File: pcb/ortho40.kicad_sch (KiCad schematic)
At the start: 128 parts, among them J1 SWD, J2 USB_C_Receptacle_USB2.0, SW1 SW_Push, U1 RP2040, U2 W25Q128JVS, U3 XC6206PxxxMR, U4 USBLC6-2SC6, Y1 12MHz

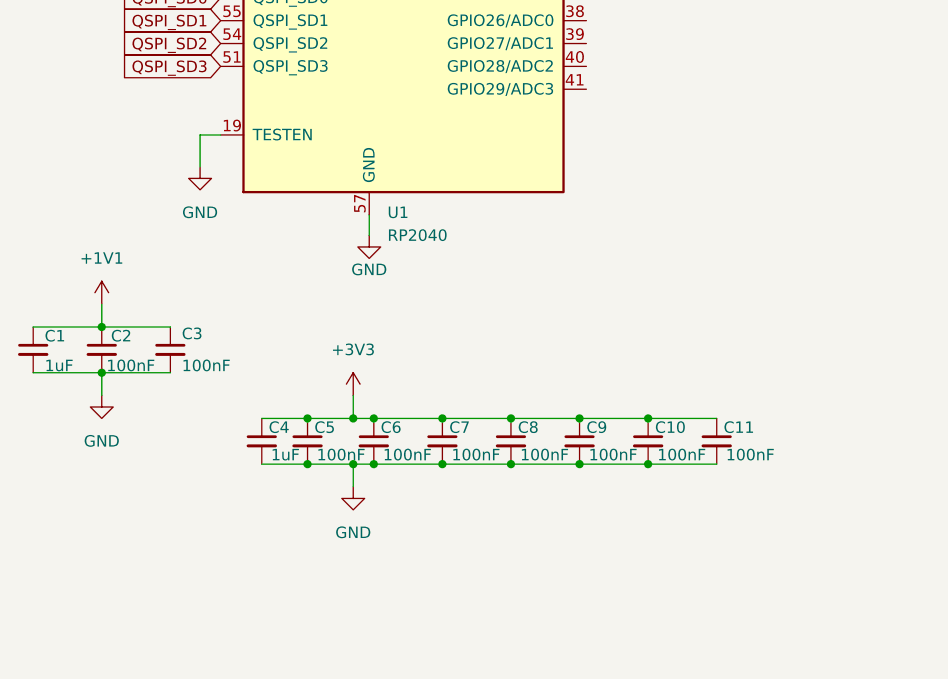
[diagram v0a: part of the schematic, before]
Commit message: blobpain
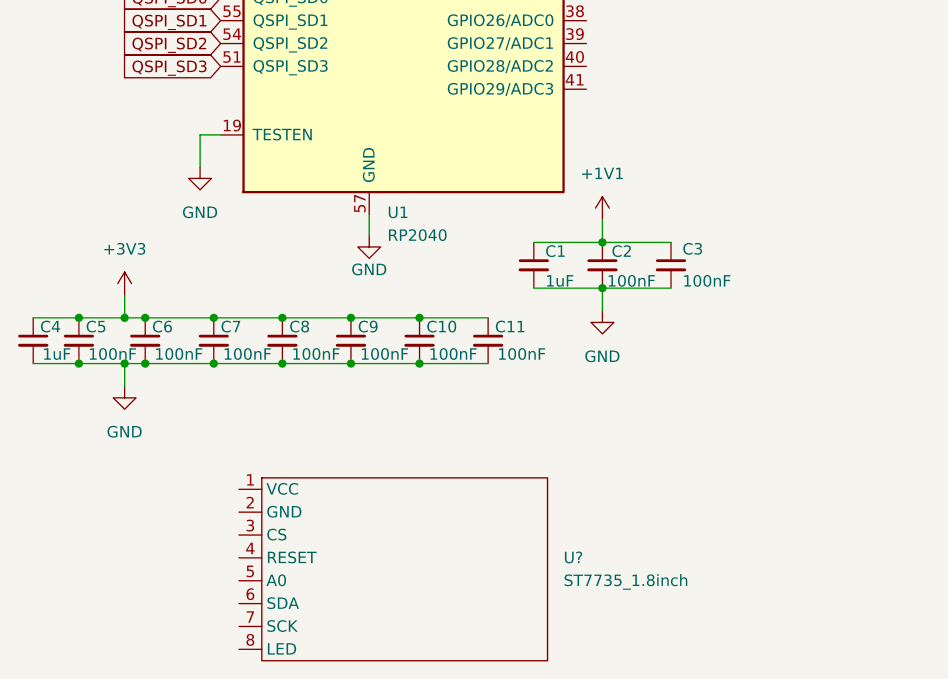
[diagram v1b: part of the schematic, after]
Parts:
- added U?: ST7735_1.8inch, symbol kicub_keyboard_extras:ST7735_1.8inch
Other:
- moved on the sheet: C1, C10, C11, C2, C3, C4, C5, C6, C7, C8, C9

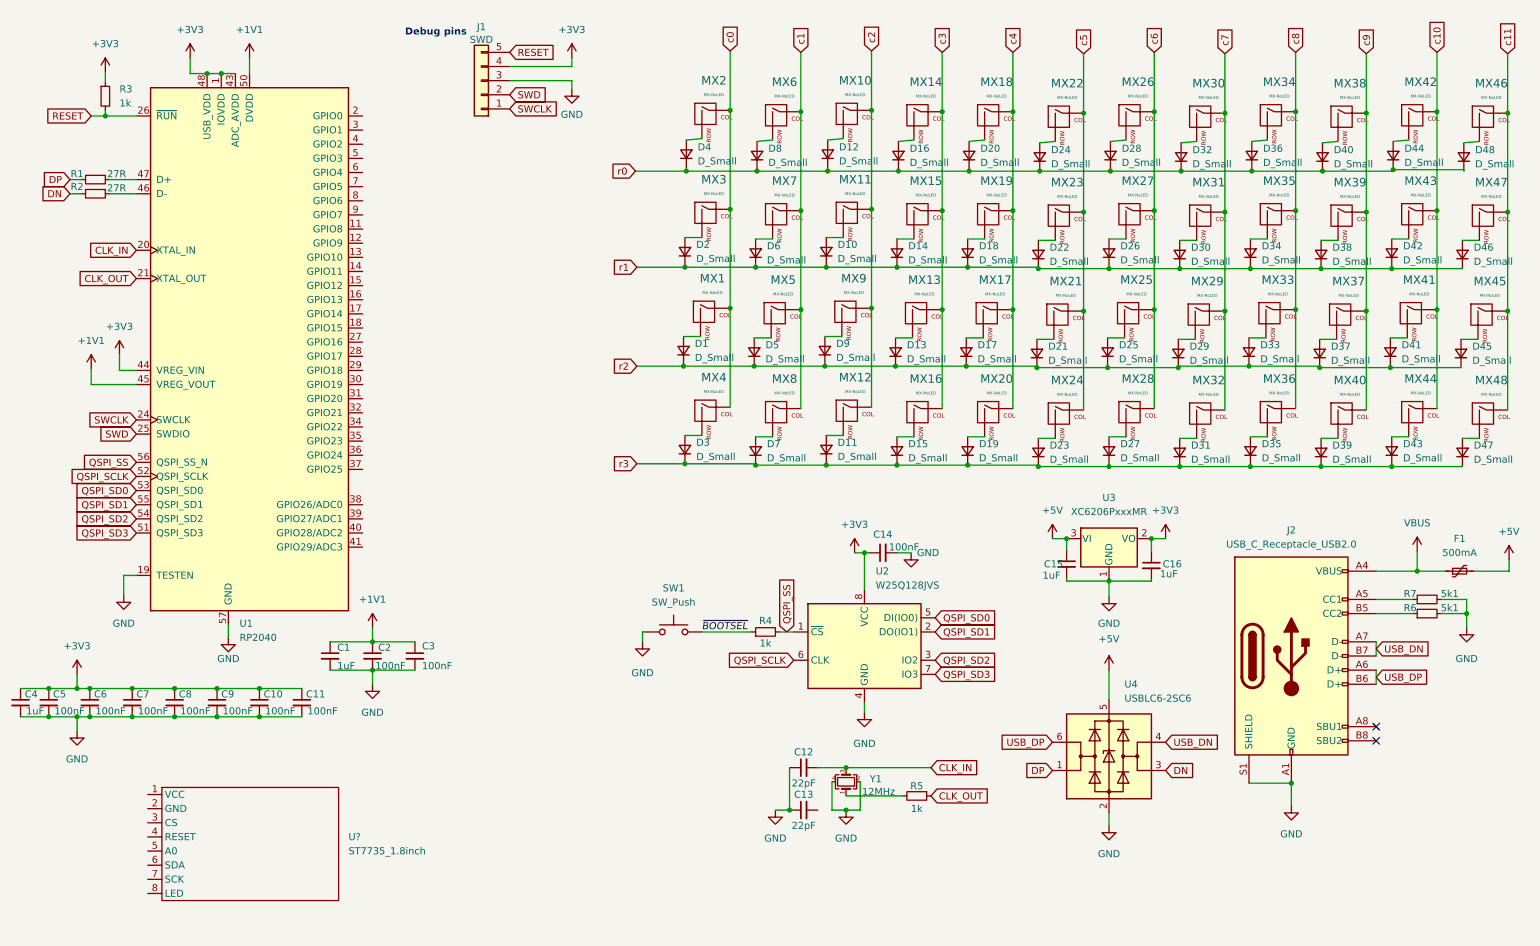
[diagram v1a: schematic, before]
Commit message: Kindof finish pcb
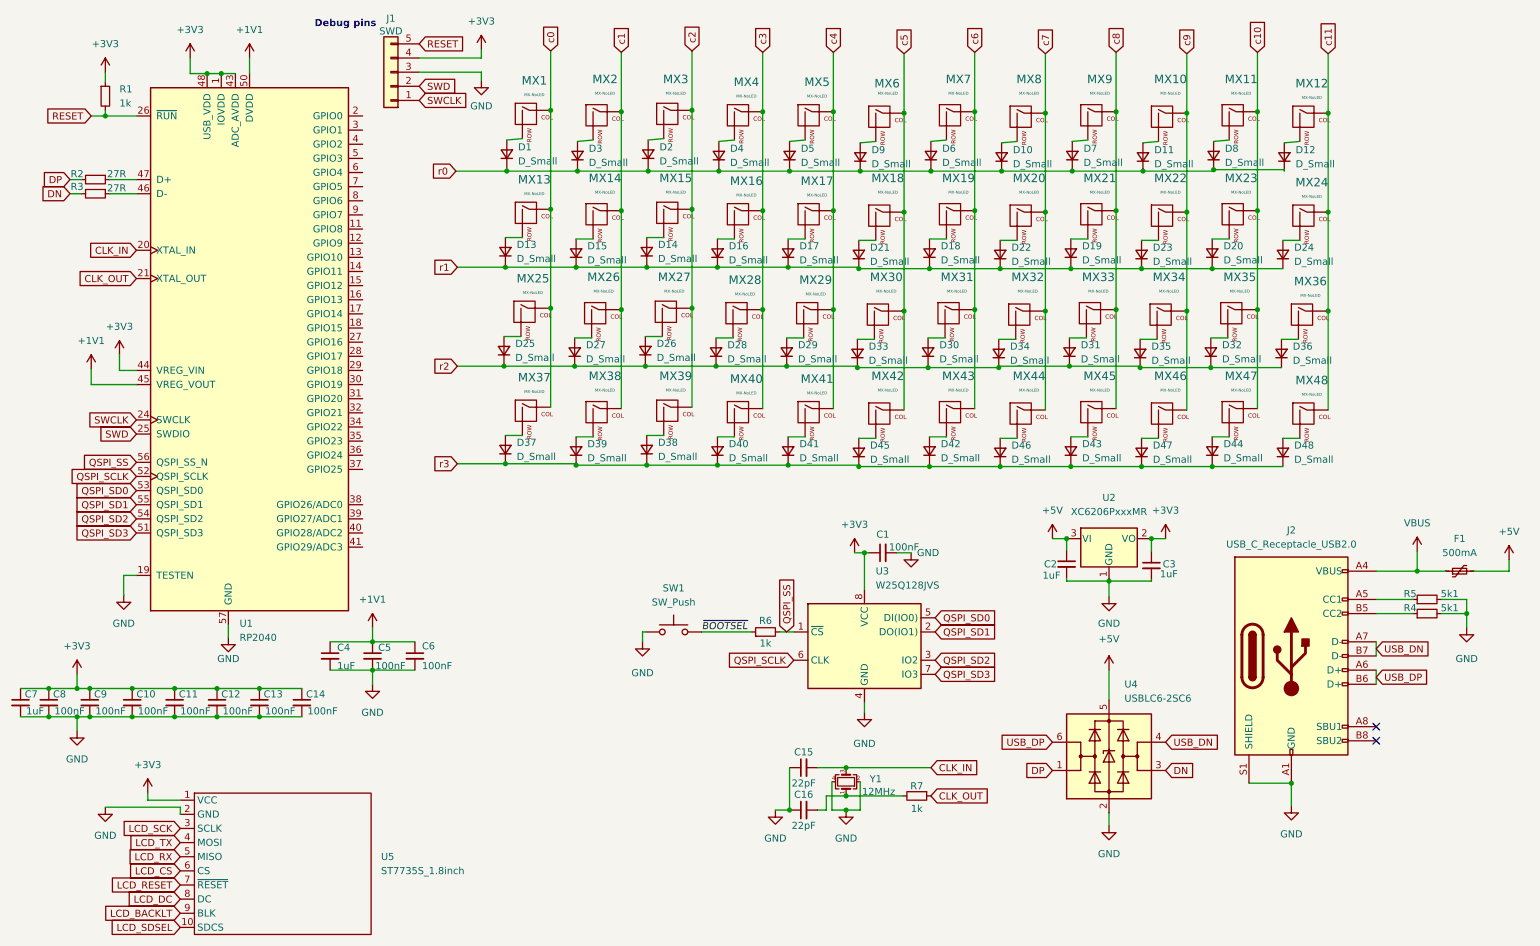
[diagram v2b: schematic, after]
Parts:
- D1: renamed from D4; footprint Diode_SMD:D_0201_0603Metric -> Diode_SMD:D_SOD-123
- D10: renamed from D32; footprint Diode_SMD:D_0201_0603Metric -> Diode_SMD:D_SOD-123
- D11: renamed from D40; footprint Diode_SMD:D_0201_0603Metric -> Diode_SMD:D_SOD-123
- D12: renamed from D48; footprint Diode_SMD:D_0201_0603Metric -> Diode_SMD:D_SOD-123
- D13: renamed from D2; footprint Diode_SMD:D_0201_0603Metric -> Diode_SMD:D_SOD-123
- D14: renamed from D10; footprint Diode_SMD:D_0201_0603Metric -> Diode_SMD:D_SOD-123
- D15: renamed from D6; footprint Diode_SMD:D_0201_0603Metric -> Diode_SMD:D_SOD-123
- D16: renamed from D14; footprint Diode_SMD:D_0201_0603Metric -> Diode_SMD:D_SOD-123
- D17: renamed from D18; footprint Diode_SMD:D_0201_0603Metric -> Diode_SMD:D_SOD-123
- D18: renamed from D26; footprint Diode_SMD:D_0201_0603Metric -> Diode_SMD:D_SOD-123
- D19: renamed from D34; footprint Diode_SMD:D_0201_0603Metric -> Diode_SMD:D_SOD-123
- D2: renamed from D12; footprint Diode_SMD:D_0201_0603Metric -> Diode_SMD:D_SOD-123
- D20: renamed from D42; footprint Diode_SMD:D_0201_0603Metric -> Diode_SMD:D_SOD-123
- D21: renamed from D22; footprint Diode_SMD:D_0201_0603Metric -> Diode_SMD:D_SOD-123
- D22: renamed from D30; footprint Diode_SMD:D_0201_0603Metric -> Diode_SMD:D_SOD-123
- D23: renamed from D38; footprint Diode_SMD:D_0201_0603Metric -> Diode_SMD:D_SOD-123
- D24: renamed from D46; footprint Diode_SMD:D_0201_0603Metric -> Diode_SMD:D_SOD-123
- D25: renamed from D1; footprint Diode_SMD:D_0201_0603Metric -> Diode_SMD:D_SOD-123
- D26: renamed from D9; footprint Diode_SMD:D_0201_0603Metric -> Diode_SMD:D_SOD-123
- D27: renamed from D5; footprint Diode_SMD:D_0201_0603Metric -> Diode_SMD:D_SOD-123
- D28: renamed from D13; footprint Diode_SMD:D_0201_0603Metric -> Diode_SMD:D_SOD-123
- D29: renamed from D17; footprint Diode_SMD:D_0201_0603Metric -> Diode_SMD:D_SOD-123
- D3: renamed from D8; footprint Diode_SMD:D_0201_0603Metric -> Diode_SMD:D_SOD-123
- D30: renamed from D25; footprint Diode_SMD:D_0201_0603Metric -> Diode_SMD:D_SOD-123
- D31: renamed from D33; footprint Diode_SMD:D_0201_0603Metric -> Diode_SMD:D_SOD-123
- D32: renamed from D41; footprint Diode_SMD:D_0201_0603Metric -> Diode_SMD:D_SOD-123
- D33: renamed from D21; footprint Diode_SMD:D_0201_0603Metric -> Diode_SMD:D_SOD-123
- D34: renamed from D29; footprint Diode_SMD:D_0201_0603Metric -> Diode_SMD:D_SOD-123
- D35: renamed from D37; footprint Diode_SMD:D_0201_0603Metric -> Diode_SMD:D_SOD-123
- D36: renamed from D45; footprint Diode_SMD:D_0201_0603Metric -> Diode_SMD:D_SOD-123
- D37: renamed from D3; footprint Diode_SMD:D_0201_0603Metric -> Diode_SMD:D_SOD-123
- D38: renamed from D11; footprint Diode_SMD:D_0201_0603Metric -> Diode_SMD:D_SOD-123
- D39: renamed from D7; footprint Diode_SMD:D_0201_0603Metric -> Diode_SMD:D_SOD-123
- D4: renamed from D16; footprint Diode_SMD:D_0201_0603Metric -> Diode_SMD:D_SOD-123
- D40: renamed from D15; footprint Diode_SMD:D_0201_0603Metric -> Diode_SMD:D_SOD-123
- D41: renamed from D19; footprint Diode_SMD:D_0201_0603Metric -> Diode_SMD:D_SOD-123
- D42: renamed from D27; footprint Diode_SMD:D_0201_0603Metric -> Diode_SMD:D_SOD-123
- D43: renamed from D35; footprint Diode_SMD:D_0201_0603Metric -> Diode_SMD:D_SOD-123
- D44: renamed from D43; footprint Diode_SMD:D_0201_0603Metric -> Diode_SMD:D_SOD-123
- D45: renamed from D23; footprint Diode_SMD:D_0201_0603Metric -> Diode_SMD:D_SOD-123
- D46: renamed from D31; footprint Diode_SMD:D_0201_0603Metric -> Diode_SMD:D_SOD-123
- D47: renamed from D39; footprint Diode_SMD:D_0201_0603Metric -> Diode_SMD:D_SOD-123
- D48: renamed from D47; footprint Diode_SMD:D_0201_0603Metric -> Diode_SMD:D_SOD-123
- D5: renamed from D20; footprint Diode_SMD:D_0201_0603Metric -> Diode_SMD:D_SOD-123
- D6: renamed from D28; footprint Diode_SMD:D_0201_0603Metric -> Diode_SMD:D_SOD-123
- D7: renamed from D36; footprint Diode_SMD:D_0201_0603Metric -> Diode_SMD:D_SOD-123
- D8: renamed from D44; footprint Diode_SMD:D_0201_0603Metric -> Diode_SMD:D_SOD-123
- D9: renamed from D24; footprint Diode_SMD:D_0201_0603Metric -> Diode_SMD:D_SOD-123
- R1: renamed from R3; footprint Resistor_SMD:R_4020_10251Metric -> Resistor_SMD:R_0402_1005Metric
- R2: renamed from R1; footprint Resistor_SMD:R_4020_10251Metric -> Resistor_SMD:R_0402_1005Metric
- R3: renamed from R2; footprint Resistor_SMD:R_4020_10251Metric -> Resistor_SMD:R_0402_1005Metric
- R4: renamed from R6; footprint Resistor_SMD:R_4020_10251Metric -> Resistor_SMD:R_0402_1005Metric
- R5: renamed from R7; footprint Resistor_SMD:R_4020_10251Metric -> Resistor_SMD:R_0402_1005Metric
- R6: renamed from R4; footprint Resistor_SMD:R_4020_10251Metric -> Resistor_SMD:R_0402_1005Metric
- R7: renamed from R5; footprint Resistor_SMD:R_4020_10251Metric -> Resistor_SMD:R_0402_1005Metric
- U5: renamed from U?; value ST7735_1.8inch -> ST7735S_1.8inch; footprint (none) -> Footprints:ST7735_1.8inch
- renumbered C14 to C1, C7 to C10, C8 to C11, C9 to C12, C10 to C13, C11 to C14, C12 to C15, C13 to C16, C15 to C2, C16 to C3, C1 to C4, C2 to C5, C3 to C6, C4 to C7, C5 to C8, C6 to C9, MX2 to MX1, MX38 to MX10, MX42 to MX11, MX46 to MX12, MX3 to MX13, MX7 to MX14, MX11 to MX15, MX15 to MX16, MX19 to MX17, MX23 to MX18, MX27 to MX19, MX6 to MX2, MX31 to MX20, MX35 to MX21, MX39 to MX22, MX43 to MX23, MX47 to MX24, MX1 to MX25, MX5 to MX26, MX9 to MX27, MX13 to MX28, MX17 to MX29, MX10 to MX3, MX21 to MX30, MX25 to MX31, MX29 to MX32, MX37 to MX34, MX41 to MX35, MX45 to MX36, MX4 to MX37, MX8 to MX38, MX12 to MX39, MX14 to MX4, MX16 to MX40, MX20 to MX41, MX24 to MX42, MX28 to MX43, MX32 to MX44, MX36 to MX45, MX40 to MX46, MX44 to MX47, MX18 to MX5, MX22 to MX6, MX26 to MX7, MX30 to MX8, MX34 to MX9, U3 to U2, U2 to U3
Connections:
- net +3V3: now also U5.1 (VCC)
- net GND: now also U5.2 (GND)
- net at R7.2, Y1.1: now also C16.2
- net LCD_SCK: now reaches U5.3 (SCLK)
- net LCD_TX: now reaches U5.4 (MOSI)
- net LCD_RX: now reaches U5.5 (MISO)
- net LCD_CS: now reaches U5.6 (CS)
- net LCD_RESET: now reaches U5.7 (~{RESET})
- net LCD_DC: now reaches U5.8 (DC)
- new net LCD_BACKLT: U5.9 (BLK)
- new net LCD_SDSEL: U5.10 (SDCS)
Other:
- moved on the sheet: D1, D10, D11, D12, D13, D14, D15, D16, D17, D18, D19, D2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
